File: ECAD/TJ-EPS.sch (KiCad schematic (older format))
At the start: 38 parts

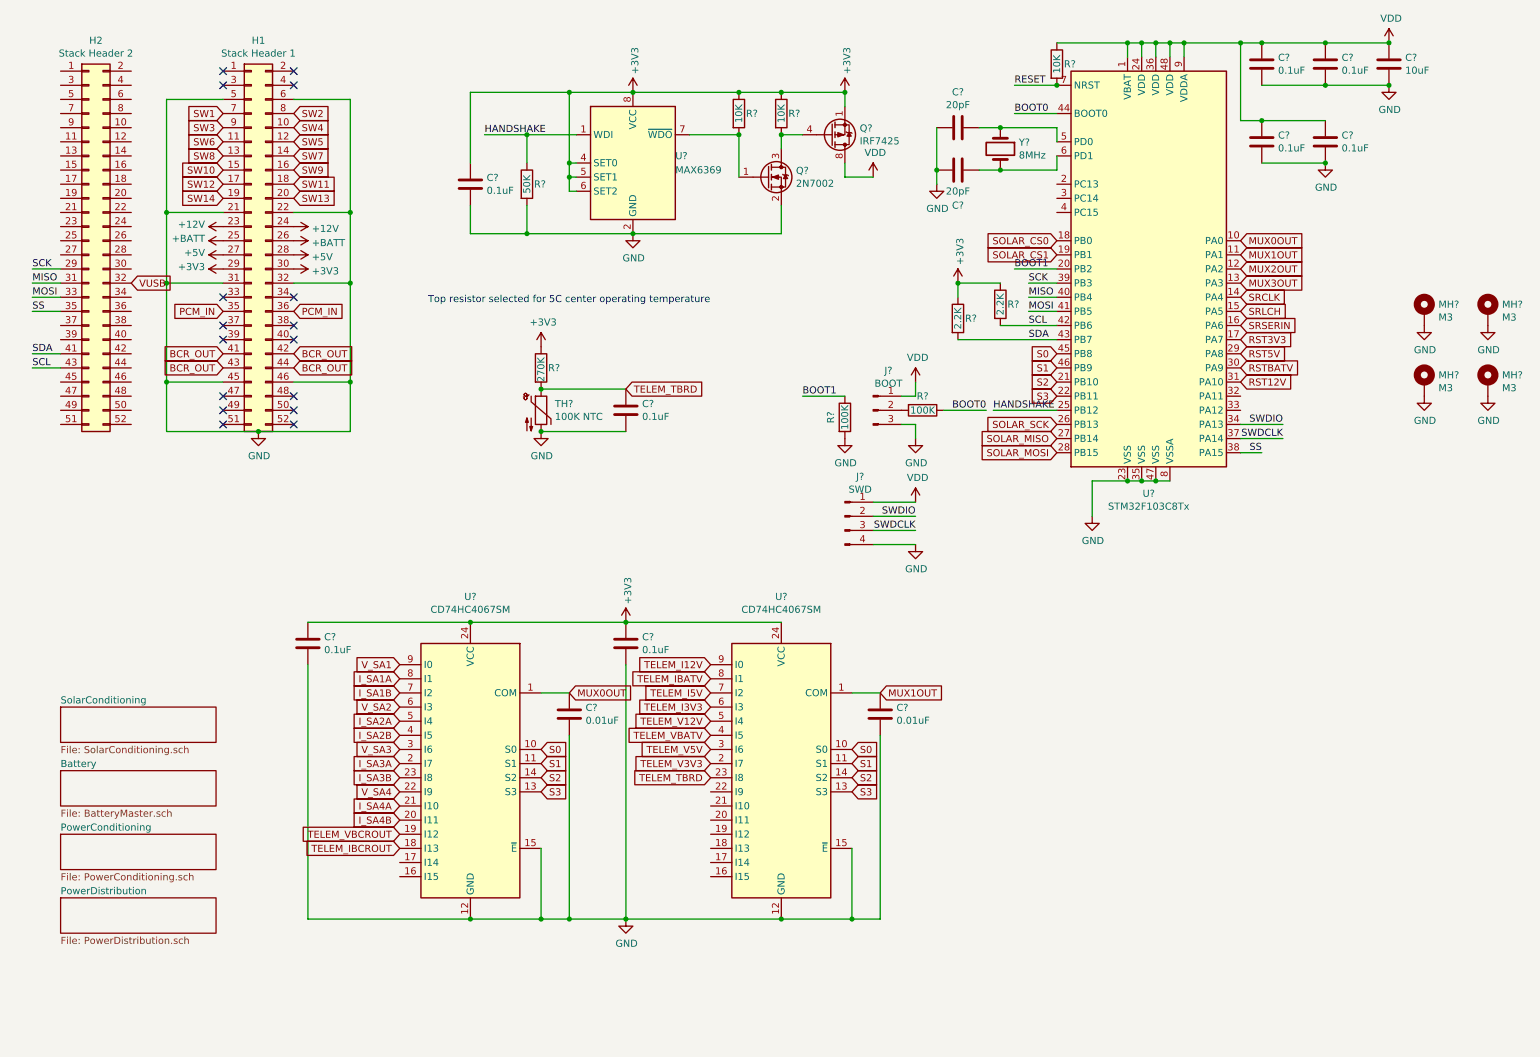
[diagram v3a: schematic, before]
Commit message: Annotate and begin adding footprints
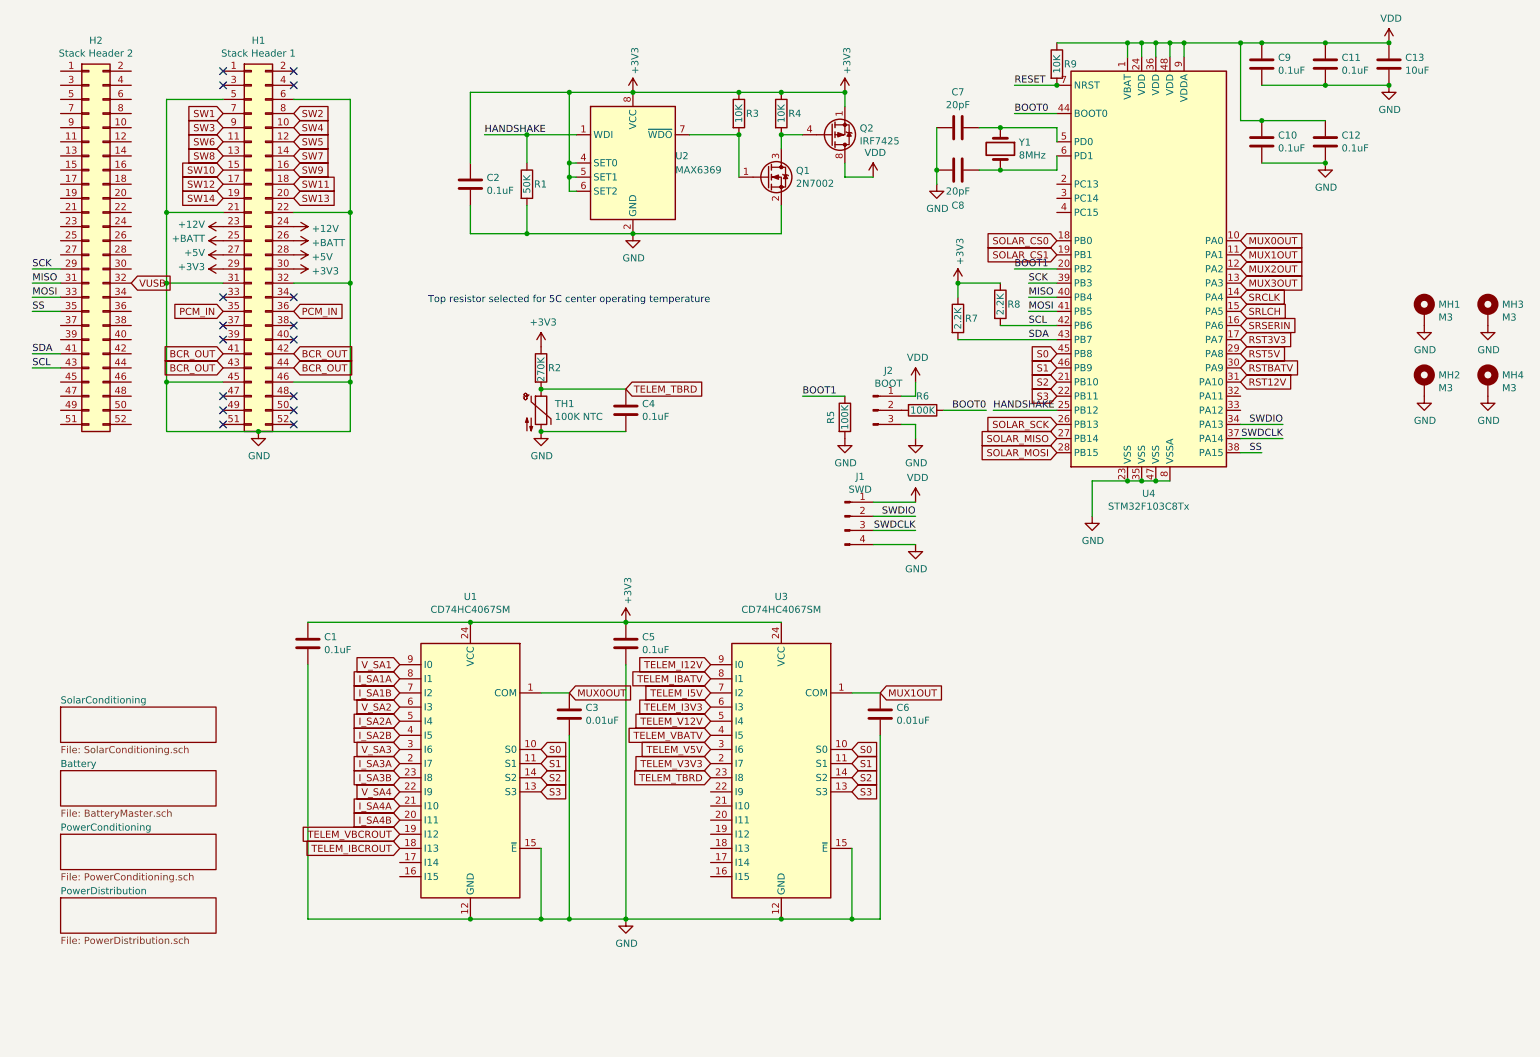
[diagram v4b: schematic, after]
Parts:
- C1, C10, C11, C12, C13, C2, C3, C4, C5, C6, C7, C8, C9: renamed from C?; footprint (none) -> Capacitor_SMD:C_0805_2012Metric
- H1, H2: footprint (none) -> Connector_PinSocket_2.54mm:PinSocket_2x26_P2.54mm_Vertical
- J1: renamed from J?; footprint (none) -> Connector_PinHeader_2.54mm:PinHeader_1x04_P2.54mm_Horizontal
- J2: renamed from J?; footprint (none) -> Connector_PinHeader_2.54mm:PinHeader_1x03_P2.54mm_Vertical
- MH1, MH2, MH3, MH4: renamed from MH?; footprint (none) -> MountingHole:MountingHole_3.2mm_M3_DIN965_Pad_TopBottom
- R1, R2, R3, R4, R5, R6, R7, R8, R9: renamed from R?; footprint (none) -> Resistor_SMD:R_0805_2012Metric
- Y1: renamed from Y?; footprint (none) -> Crystal:Crystal_HC49-4H_Vertical
- gave numbers to parts that had none: 7

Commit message: Add all IC footprints
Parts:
- TH1: footprint (none) -> Resistor_SMD:R_1206_3216Metric
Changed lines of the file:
@@
 F 0 "TH1" H 4248 3396 50  0000 L CNN
 F 1 "100K NTC" H 4248 3305 50  0000 L CNN
-F 2 "" H 4150 3400 50  0001 C CNN
+F 2 "Resistor_SMD:R_1206_3216Metric" H 4150 3400 50  0001 C CNN
 F 3 "~" H 4150 3400 50  0001 C CNN
 	1    4150 3350

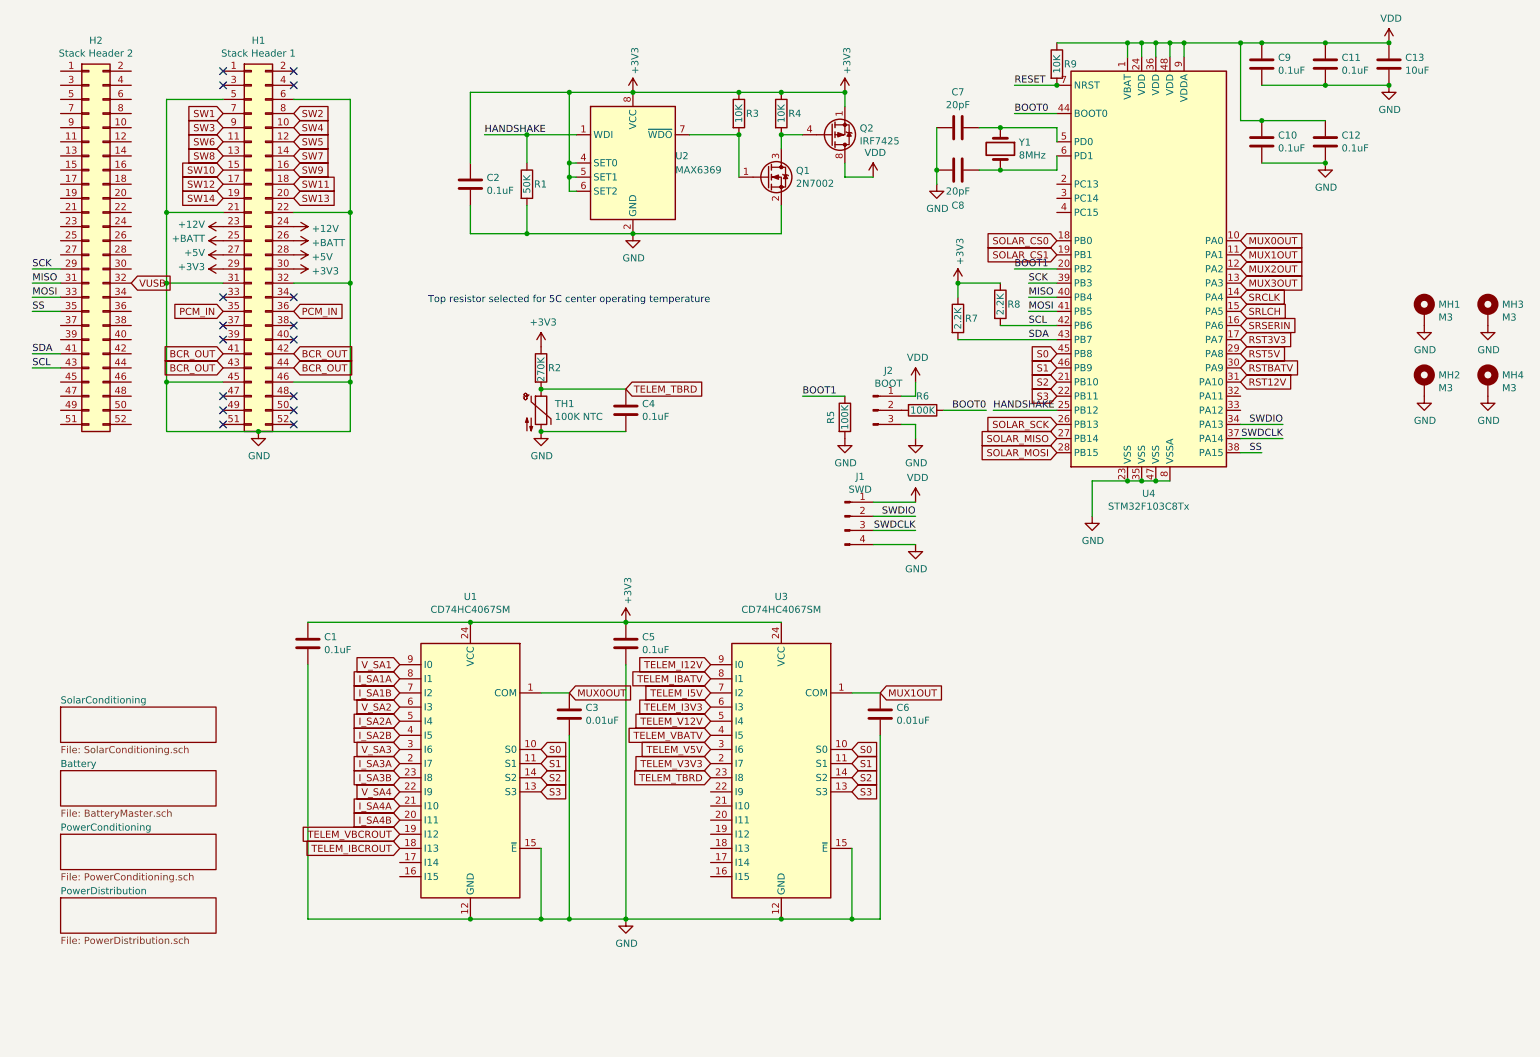
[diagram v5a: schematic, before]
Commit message: Major descope, remove 12V boost and all related circuitry
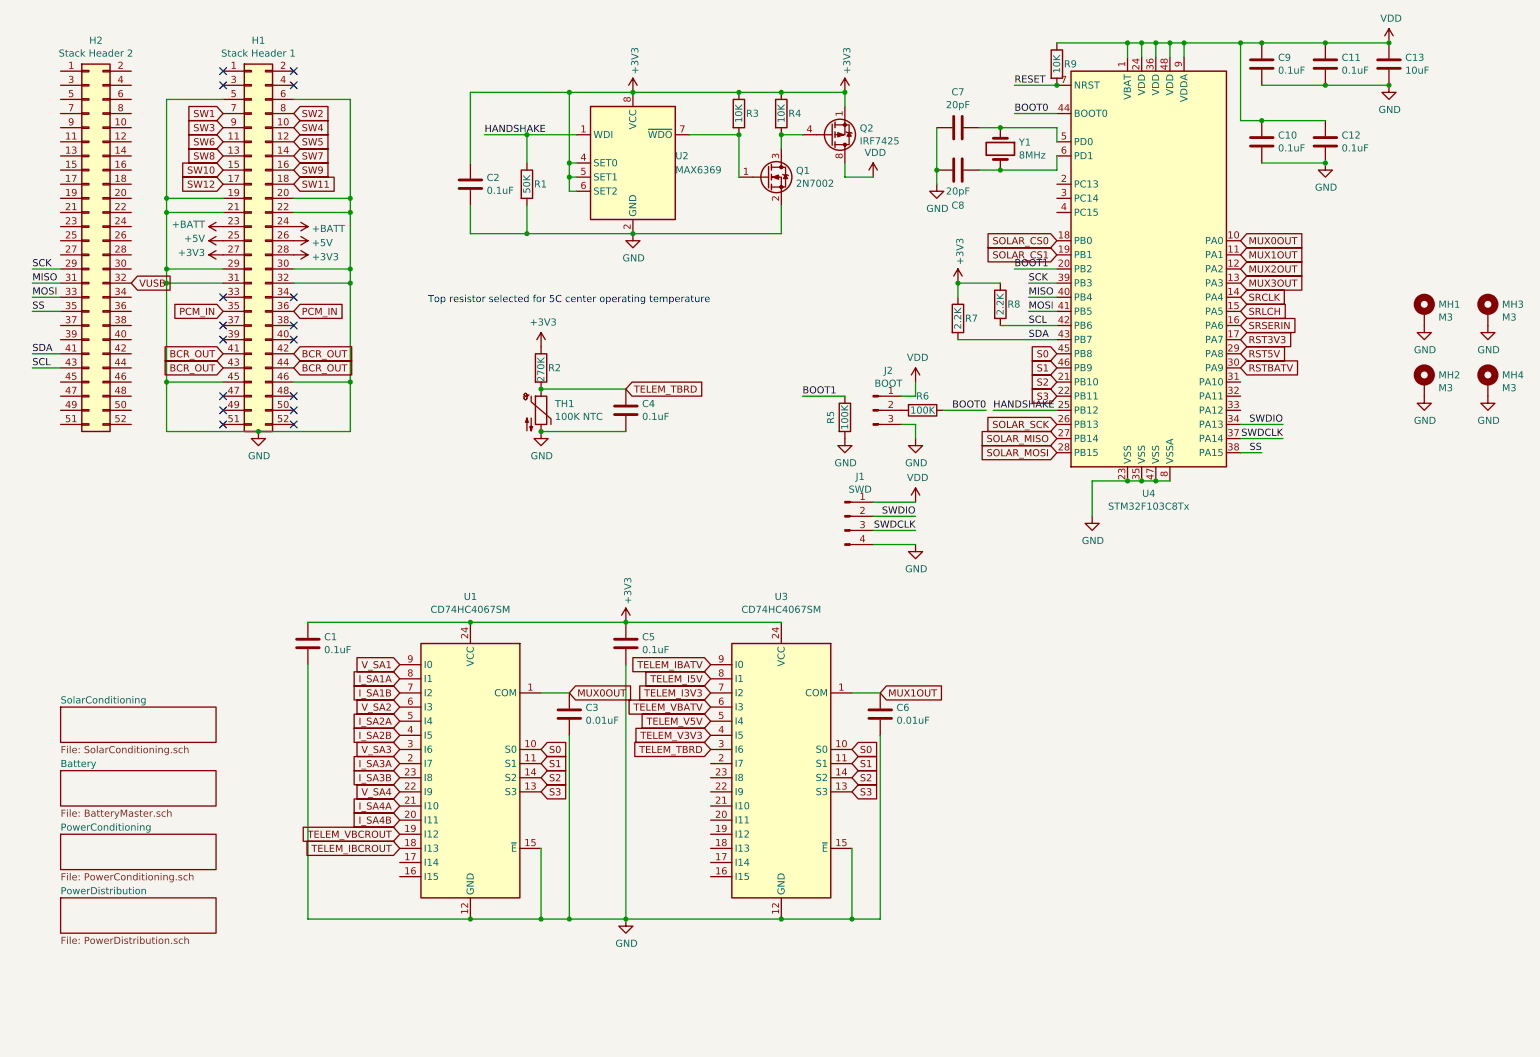
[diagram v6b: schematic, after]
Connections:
- net +12V is gone; now on net +BATT: H1.23 (Pin_23), H1.24 (Pin_24)
- net SW13 is gone; now on net GND: H1.20 (Pin_20)
- net SW14 is gone; now on net GND: H1.19 (Pin_19)
- net TELEM_I12V is gone; now on net TELEM_IBATV: U3.9 (I0)
- net TELEM_V12V is gone; now on net TELEM_V5V: U3.5 (I4)
- net +3V3: now also H1.27 (Pin_27), H1.28 (Pin_28); no longer H1.29 (Pin_29), H1.30 (Pin_30)
- net +5V: now also H1.25 (Pin_25), H1.26 (Pin_26); no longer H1.27 (Pin_27), H1.28 (Pin_28)
- net +BATT: no longer H1.25 (Pin_25), H1.26 (Pin_26)
- net GND: now also H1.29 (Pin_29), H1.30 (Pin_30)
- net TELEM_I3V3: now also U3.7 (I2); no longer U3.6 (I3)
- net TELEM_I5V: now also U3.8 (I1); no longer U3.7 (I2)
- net TELEM_IBATV: no longer U3.8 (I1)
- net TELEM_TBRD: now also U3.3 (I6); no longer U3.23 (I8)
- net TELEM_V3V3: now also U3.4 (I5); no longer U3.2 (I7)
- net TELEM_V5V: no longer U3.3 (I6)
- net TELEM_VBATV: now also U3.6 (I3); no longer U3.4 (I5)
- net RST12V: no longer names the net of U4.31 (PA10)
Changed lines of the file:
@@
 $Descr A4 11693 8268
 encoding utf-8
-Sheet 1 44
+Sheet 1 37
 Title "TJ Custom EPS"
 Date ""
@@
 SW10
 $Comp
-L power:+12V #PWR0101
-U 1 1 61BC2B50
-P 2400 2050
-F 0 "#PWR0101" H 2400 1900 50  0001 C CNN
-F 1 "+12V" V 2415 2178 50  0000 L CNN
-F 2 "" H 2400 2050 50  0001 C CNN
-F 3 "" H 2400 2050 50  0001 C CNN
-	1    2400 2050
-	0    1    1    0
-$EndComp
-$Comp
-L power:+12V #PWR0102
-U 1 1 61BC30BA
-P 1900 2050
-F 0 "#PWR0102" H 1900 1900 50  0001 C CNN
-F 1 "+12V" V 1915 2178 50  0000 L CNN
-F 2 "" H 1900 2050 50  0001 C CNN
-F 3 "" H 1900 2050 50  0001 C CNN
-	1    1900 2050
-	0    -1   -1   0
-$EndComp
-$Comp
 L power:+5V #PWR0103
 U 1 1 61BC34F8
+P 1900 2150
+F 0 "#PWR0103" H 1900 2000 50  0001 C CNN
+F 1 "+5V" V 1915 2278 50  0000 L CNN
+F 2 "" H 1900 2150 50  0001 C CNN
+F 3 "" H 1900 2150 50  0001 C CNN
+	1    1900 2150
+	0    -1   -1   0
+$EndComp
+$Comp
+L power:+5V #PWR0104
+U 1 1 61BC3941
+P 2400 2150
+F 0 "#PWR0104" H 2400 2000 50  0001 C CNN
+F 1 "+5V" V 2415 2278 50  0000 L CNN
+F 2 "" H 2400 2150 50  0001 C CNN
+F 3 "" H 2400 2150 50  0001 C CNN
+	1    2400 2150
+	0    1    1    0
+$EndComp
+$Comp
+L power:+3V3 #PWR0105
+U 1 1 61BC3DF9
 P 1900 2250
-F 0 "#PWR0103" H 1900 2100 50  0001 C CNN
-F 1 "+5V" V 1915 2378 50  0000 L CNN
+F 0 "#PWR0105" H 1900 2100 50  0001 C CNN
+F 1 "+3V3" V 1915 2378 50  0000 L CNN
 F 2 "" H 1900 2250 50  0001 C CNN
 F 3 "" H 1900 2250 50  0001 C CNN
@@
 $EndComp
 $Comp
-L power:+5V #PWR0104
-U 1 1 61BC3941
+L power:+3V3 #PWR0106
+U 1 1 61BC42A2
 P 2400 2250
-F 0 "#PWR0104" H 2400 2100 50  0001 C CNN
-F 1 "+5V" V 2415 2378 50  0000 L CNN
+F 0 "#PWR0106" H 2400 2100 50  0001 C CNN
+F 1 "+3V3" V 2415 2378 50  0000 L CNN
 F 2 "" H 2400 2250 50  0001 C CNN
 F 3 "" H 2400 2250 50  0001 C CNN
 	1    2400 2250
-	0    1    1    0
-$EndComp
-$Comp
-L power:+3V3 #PWR0105
-U 1 1 61BC3DF9
-P 1900 2350
-F 0 "#PWR0105" H 1900 2200 50  0001 C CNN
-F 1 "+3V3" V 1915 2478 50  0000 L CNN
-F 2 "" H 1900 2350 50  0001 C CNN
-F 3 "" H 1900 2350 50  0001 C CNN
-	1    1900 2350
-	0    -1   -1   0
-$EndComp
-$Comp
-L power:+3V3 #PWR0106
-U 1 1 61BC42A2
-P 2400 2350
-F 0 "#PWR0106" H 2400 2200 50  0001 C CNN
-F 1 "+3V3" V 2415 2478 50  0000 L CNN
-F 2 "" H 2400 2350 50  0001 C CNN
-F 3 "" H 2400 2350 50  0001 C CNN
-	1    2400 2350
 	0    1    1    0
 $EndComp
@@
 L power:+BATT #PWR0107
 U 1 1 61BC5790
-P 2400 2150
-F 0 "#PWR0107" H 2400 2000 50  0001 C CNN
-F 1 "+BATT" V 2415 2278 50  0000 L CNN
-F 2 "" H 2400 2150 50  0001 C CNN
-F 3 "" H 2400 2150 50  0001 C CNN
-	1    2400 2150
+P 2400 2050
+F 0 "#PWR0107" H 2400 1900 50  0001 C CNN
+F 1 "+BATT" V 2415 2178 50  0000 L CNN
+F 2 "" H 2400 2050 50  0001 C CNN
+F 3 "" H 2400 2050 50  0001 C CNN
+	1    2400 2050
 	0    1    1    0
 $EndComp
@@
 L power:+BATT #PWR0108
 U 1 1 61BC64DC
-P 1900 2150
-F 0 "#PWR0108" H 1900 2000 50  0001 C CNN
-F 1 "+BATT" V 1915 2278 50  0000 L CNN
-F 2 "" H 1900 2150 50  0001 C CNN
-F 3 "" H 1900 2150 50  0001 C CNN
-	1    1900 2150
+P 1900 2050
+F 0 "#PWR0108" H 1900 1900 50  0001 C CNN
+F 1 "+BATT" V 1915 2178 50  0000 L CNN
+F 2 "" H 1900 2050 50  0001 C CNN
+F 3 "" H 1900 2050 50  0001 C CNN
+	1    1900 2050
 	0    -1   -1   0
 $EndComp
@@
 Text GLabel 2400 1750 2    50   Input ~ 0
 SW11
-Text GLabel 2400 1850 2    50   Input ~ 0
-SW13
 Text GLabel 1900 1750 0    50   Input ~ 0
 SW12
-Text GLabel 1900 1850 0    50   Input ~ 0
-SW14
 $Comp
 L Connector_Generic:Conn_02x26_Odd_Even H1
@@
 	2800 1150 2400 1150
 Wire Wire Line
-	2800 1150 2800 1950
+	2800 1150 2800 1850
 Wire Wire Line
 	1900 1150 1500 1150
 Wire Wire Line
-	1500 1150 1500 1950
+	1500 1150 1500 1850
 Connection ~ 1500 2450
 Wire Wire Line
 	1500 2450 1500 3150
-Wire Wire Line
-	1500 1950 1500 2450
 Connection ~ 2800 2450
 Wire Wire Line
 	2800 2450 2800 3150
-Wire Wire Line
-	2800 1950 2800 2450
 Connection ~ 2800 3150
 Wire Wire Line
@@
 TELEM_IBCROUT
 Text GLabel 5350 5150 0    50   Input ~ 0
-TELEM_I12V
+TELEM_IBATV
 Text GLabel 5350 5250 0    50   Input ~ 0
-TELEM_IBATV
+TELEM_I5V
 Text GLabel 5350 5350 0    50   Input ~ 0
-TELEM_I5V
+TELEM_I3V3
 Text GLabel 5350 5450 0    50   Input ~ 0
-TELEM_I3V3
+TELEM_VBATV
 Text GLabel 5350 5550 0    50   Input ~ 0
-TELEM_V12V
+TELEM_V5V
 Text GLabel 5350 5650 0    50   Input ~ 0
-TELEM_VBATV
-Text GLabel 5350 5750 0    50   Input ~ 0
-TELEM_V5V
-Text GLabel 5350 5850 0    50   Input ~ 0
 TELEM_V3V3
 $Comp
@@
 	-1   0    0    -1
 $EndComp
-Text GLabel 5350 5950 0    50   Input ~ 0
+Text GLabel 5350 5750 0    50   Input ~ 0
 TELEM_TBRD
 Text GLabel 7800 3450 0    50   Input ~ 0
@@
 Text GLabel 9100 2450 2    50   Input ~ 0
 MUX3OUT
-Text GLabel 9100 3150 2    50   Input ~ 0
-RST12V
 Text GLabel 9100 3050 2    50   Input ~ 0
 RSTBATV
@@
 Text GLabel 9100 2750 2    50   Input ~ 0
 SRSERIN
+Wire Wire Line
+	2400 2350 2800 2350
+Wire Wire Line
+	1900 2350 1500 2350
+Wire Wire Line
+	2400 1850 2800 1850
+Connection ~ 2800 1850
+Wire Wire Line
+	2800 1850 2800 1950
+Wire Wire Line
+	1900 1850 1500 1850
+Connection ~ 1500 1850
+Wire Wire Line
+	1500 1850 1500 1950
+Wire Wire Line
+	2800 1950 2800 2350
+Wire Wire Line
+	1500 1950 1500 2350
+Connection ~ 2800 2350
+Wire Wire Line
+	2800 2350 2800 2450
+Connection ~ 1500 2350
+Wire Wire Line
+	1500 2350 1500 2450
 $EndSCHEMATC
